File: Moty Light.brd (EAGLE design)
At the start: 64 x 40 mm, 21 parts, among them T1 BTA16

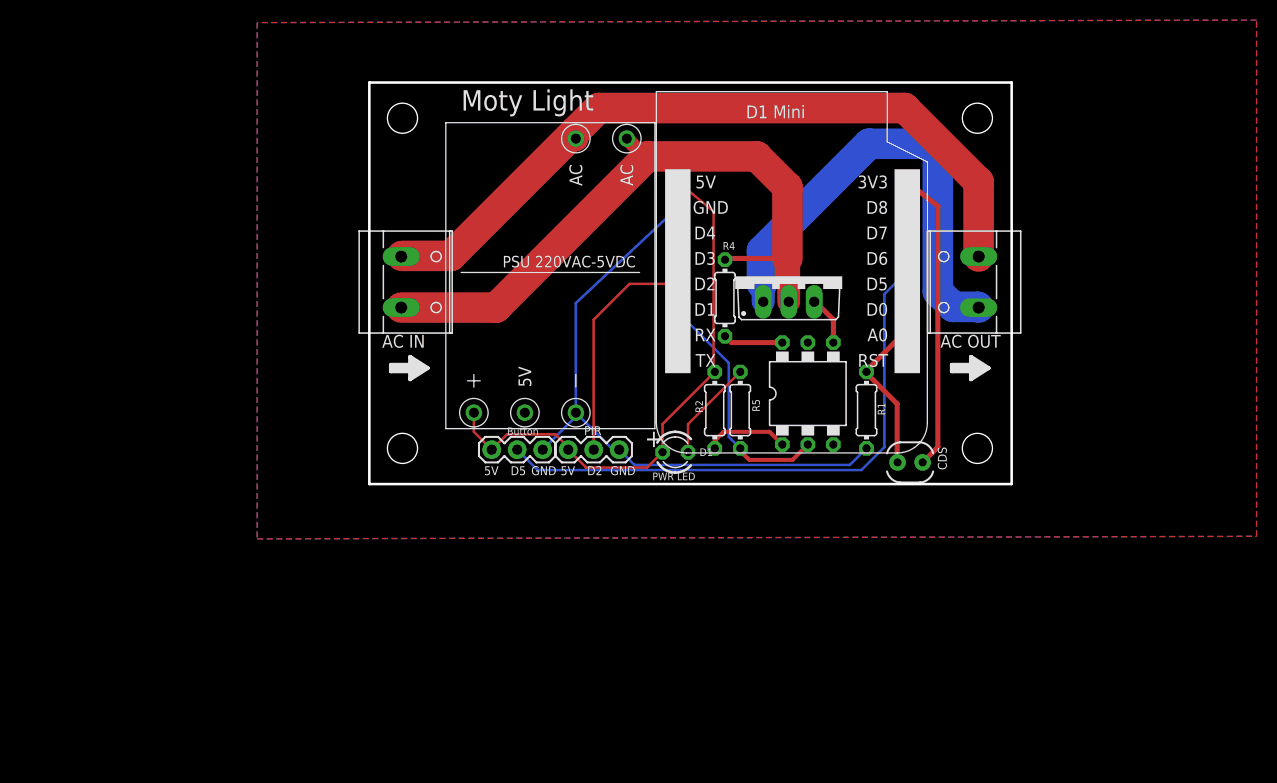
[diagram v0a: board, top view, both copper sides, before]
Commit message: Update to version 0.2
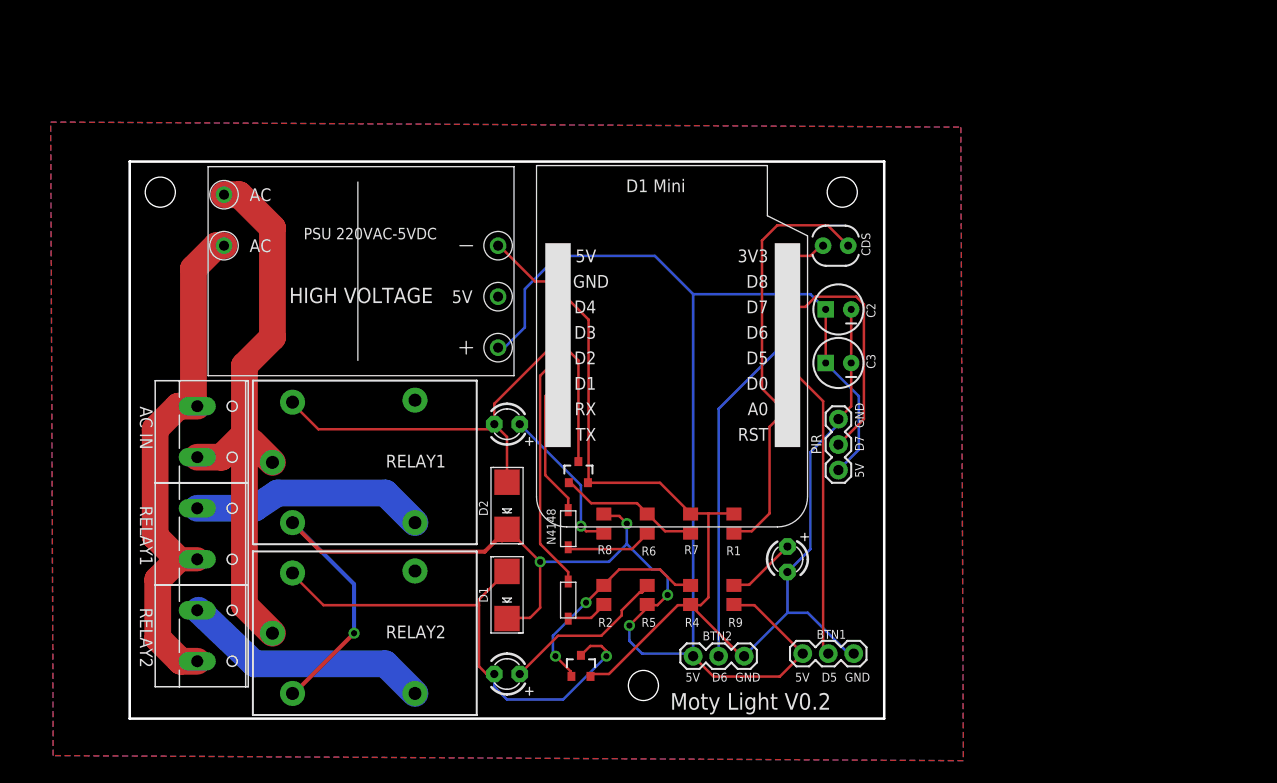
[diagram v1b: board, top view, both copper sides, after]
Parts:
- removed AC_OUT: (no value), con-wago-508:W237-132
- removed BUTTON: Button, SparkFun-Connectors:1X03
- removed OK1: MOC3041, optocoupler:DIL06B
- removed T1: BTA16, triac:TO220BV
- removed U$1, U$2: (no value), dicons:ICON_ARROW-S
- removed U$6: (no value), penn-engineering:KFH-M3
- added AC1, AC2: (no value), con-wago-508:W237-132
- added BTN2: BTN2, SparkFun-Connectors:1X03
- added BUTTON1: BTN1, SparkFun-Connectors:1X03
- added C1, C1815: C1815, SparkFun-DiscreteSemi:SOT23-3
- added C2: 47uF/16V, SparkFun-Capacitors:CPOL-RADIAL-10UF-25V
- added C3: 102pF, SparkFun-Capacitors:CPOL-RADIAL-10UF-25V
- added D2: (no value), adafruit:SMADIODE
- added N1: N4148, adafruit:SOD-123
- added N4148: (no value), adafruit:SOD-123
- added PWR_LED: PWR, adafruit:LED3MM
- added R6, R8, R9: 1K, rcl:R0805
- added R7: 4.7K, rcl:R0805
- added RELAY1, RELAY2: ZNS5106, relay:ZN5
- added RELAY_LED1: RELAY1, adafruit:LED3MM
- added RELAY_LED2: Relay2, adafruit:LED3MM
- D1: device led:LED3MM -> adafruit:SMADIODE
- R1: device rcl:0204/7 -> rcl:R0805
- R2, R5: value 330 -> 1K; device rcl:0204/7 -> rcl:R0805
- R4: value 180 -> 4.7K; device rcl:0204/7 -> rcl:R0805
- moved U$7 40.8 mm to (52.2, 10.8)
- moved R4 29.8 mm to (56.9, 19.8)
- moved U$9 25.2 mm to (4.06, 59.9)
- moved AC 25.2 mm to (8.38, 36.1)
- moved R3 22.9 mm to (71.2, 54.6), turned to 0 degrees
- moved PIR 22.1 mm to (71.6, 37.3), turned to 270 degrees
- moved D1 22.0 mm to (38.6, 19.8), turned to 90 degrees
- moved R2 21.5 mm to (48.3, 19.8), turned to 90 degrees
- moved R5 20.6 mm to (52.6, 19.8), turned to 90 degrees
- moved U$17 19.8 mm to (23.9, 45.0)
- moved U$3 19.2 mm to (23.7, 52.1), turned to 0 degrees
- moved R1 17.4 mm to (61.2, 26.9), turned to 270 degrees
- moved U$8 15.3 mm to (72.0, 59.9)
- moved U$10 14.0 mm to (66.5, 53.6)
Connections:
- removed net AC_L: AC.2, R4.2, T1.T2, U$3.J1.1
- removed net AC_N: AC.1, AC_OUT.2, U$3.J1.2
- removed net N$14: OK1.6, R4.1
- removed net N$23: AC_OUT.1, T1.T1
- removed net N$28: D1.K, R5.1
- new net HOT: AC.2, RELAY1.11, RELAY2.11, U$3.J1.1
- new net N$1: C1815.3, D2.A, RELAY1.A2, RELAY_LED1.K
- new net N$3: N4148.C, R6.1
- new net N$4: R8.2, RELAY_LED1.A
- new net N$5: C1.3, D1.A, RELAY2.A2, RELAY_LED2.K
- new net N$6: C1.1, R2.2, R4.2
- new net N$7: C1815.1, R6.2, R7.2
- new net N$8: N1.C, R2.1
- new net NC1: RELAY1.12
- new net NC2: RELAY2.12
- new net NEUTRAL: AC.1, AC1.2, AC2.2, U$3.J1.2
- new net NO1: AC1.1, RELAY1.14
- new net NO2: AC2.1, RELAY2.14
- net 5V: now also BTN2.3, BUTTON1.3, C2.1, C3.1, D1.C, D2.C, R5.1, R8.1, R9.1, RELAY1.A1, RELAY2.A1; no longer BUTTON.3, D1.A, R2.1
- net D1: now also N4148.A; no longer OK1.2, R5.2
- net D2: now also N1.A; no longer PIR.2
- net D5: now also BUTTON1.2; no longer BUTTON.2
- net D6: now also BTN2.2
- net D7: now also PIR.2
- net GND: now also BTN2.1, BUTTON1.1, C1.2, C1815.2, C2.2, C3.2, PWR_LED.K, R4.1, R7.1; no longer BUTTON.1
- net N$10: now also PWR_LED.A, R9.2; no longer OK1.1, R2.2
- net N$9: now also R5.2, RELAY_LED2.A; no longer OK1.4, T1.G
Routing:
- net 5V: track 55.0 -> 212.6 mm, vias 0 -> 5
- net AC_N: track 74.9 -> 0.00 mm
- net AC_L: track 66.5 -> 0.00 mm
- net GND: track 61.7 -> 122.9 mm
- net HOT: track 0.00 -> 58.0 mm
- net NEUTRAL: track 0.00 -> 52.4 mm
- net N$1: track 0.00 -> 51.3 mm
- net N$5: track 0.00 -> 50.8 mm, vias 0 -> 1
- net N$23: track 45.9 -> 0.00 mm
- net D6: track 0.00 -> 35.1 mm
- net A0: track 16.7 -> 43.8 mm
- net 3V3: track 30.0 -> 3.97 mm
- net D5: track 56.9 -> 31.1 mm
- net NO2: track 0.00 -> 25.1 mm
- net D7: track 0.00 -> 23.4 mm
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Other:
- board size 64 x 40 mm -> 75.2 x 55.5 mm
- board text added: "D6"
- board text added: "D7"
- board text added: "Moty Light V0.2"
- board text added: "RELAY1"
- board text added: "RELAY2"
- board text removed: "+"
- board text removed: "AC OUT"
- board text removed: "D2"
- board text removed: "Moty Light"
- board text removed: "PWR LED"

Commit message: Update design to version 0.3
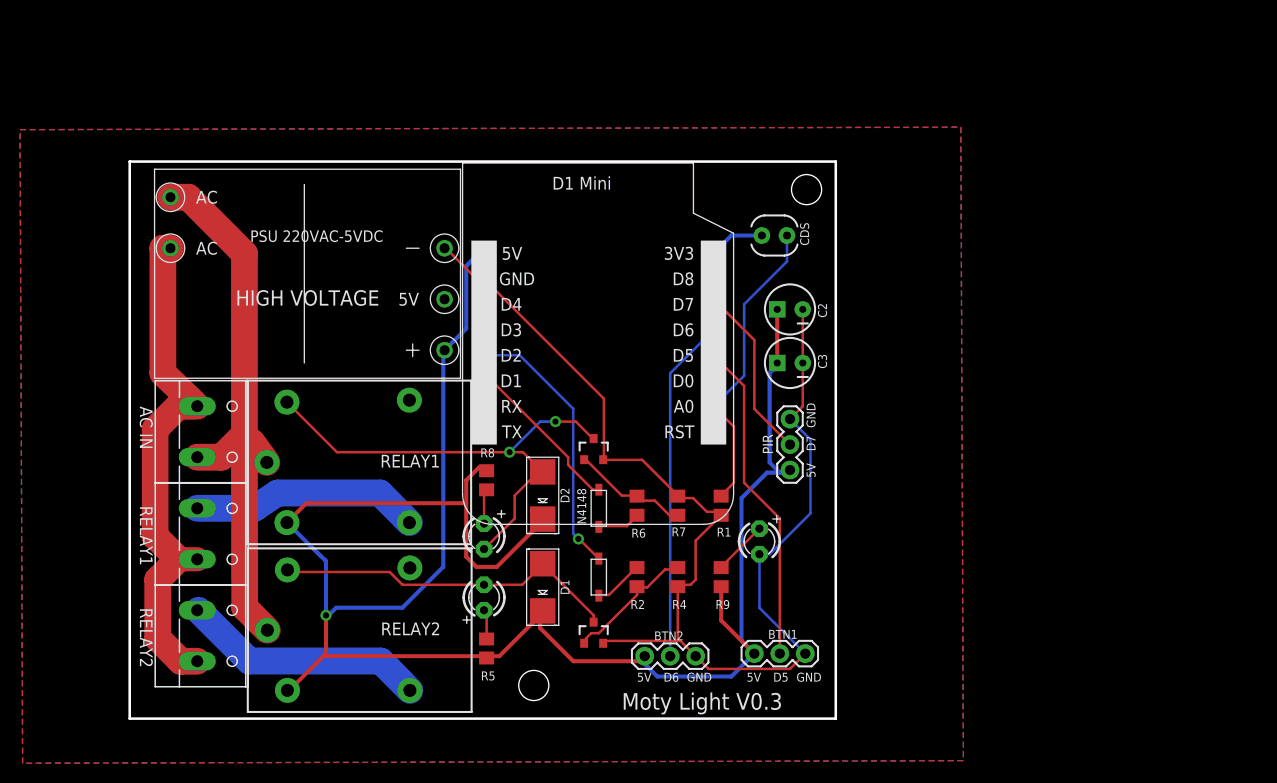
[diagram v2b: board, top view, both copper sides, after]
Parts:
- removed C1, C1815: C1815, SparkFun-DiscreteSemi:SOT23-3
- removed U$9: (no value), penn-engineering:KFH-M3
- added Q1, Q2: C1815, SparkFun-DiscreteSemi:SOT23-3
- RELAY_LED1: value RELAY1 -> Relay1
- moved R5 16.9 mm to (36.6, 14.5)
- moved R8 12.5 mm to (36.6, 31.2)
- moved RELAY_LED1 11.4 mm to (36.3, 25.7), turned to 270 degrees
- moved U$7 10.9 mm to (41.3, 10.8)
- moved RELAY_LED2 7.96 mm to (36.3, 19.6), turned to 90 degrees
- moved U$10 7.37 mm to (59.2, 53.8)
- moved R3 6.18 mm to (65.2, 55.6)
- moved U$17 5.34 mm to (18.5, 44.7)
- moved U$3 5.34 mm to (18.4, 51.8)
- moved BUTTON1 4.83 mm to (68.3, 14.0)
- moved BTN2 4.83 mm to (57.4, 13.7)
- moved C2 4.83 mm to (66.8, 48.3)
- moved C3 4.83 mm to (66.8, 42.9)
- moved PIR 4.83 mm to (66.8, 37.3)
- moved N1 3.81 mm to (47.8, 21.6)
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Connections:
- net GND: now also Q1.2, Q2.2; no longer C1.2, C1815.2
- net N$1: now also Q1.3; no longer C1815.3
- net N$5: now also Q2.3; no longer C1.3
- net N$6: now also Q2.1; no longer C1.1
- net N$7: now also Q1.1; no longer C1815.1
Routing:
- net N$5: track 50.8 -> 34.9 mm, vias 1 -> 0
- net N$9: track 16.8 -> 2.92 mm
- net A0: track 43.8 -> 30.4 mm
- net N$4: track 15.4 -> 3.98 mm, vias 1 -> 0
- net N$6: track 22.0 -> 13.3 mm, vias 2 -> 0
- net 5V: track 212.6 -> 204.6 mm, vias 5 -> 1
- net D7: track 23.4 -> 17.4 mm
- net N$3: track 8.75 -> 4.37 mm
- net GND: track 122.9 -> 119.8 mm
- net D2: track 24.2 -> 27.1 mm, vias 0 -> 1
- net N$7: track 14.4 -> 11.9 mm
- net D1: track 14.1 -> 16.6 mm
- net N$1: track 51.3 -> 49.4 mm, vias 0 -> 2
- net 3V3: track 3.97 -> 5.56 mm
- net N$10: track 6.98 -> 5.45 mm
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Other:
- board size 75.2 x 55.5 mm -> 70.3 x 55.5 mm
- board text added: "Moty Light V0.3"
- board text removed: "Moty Light V0.2"
